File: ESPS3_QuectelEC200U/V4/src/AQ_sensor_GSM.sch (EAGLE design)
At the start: 160 parts, among them J1 F-1X03-SIP-100-32, J2 53261-0871, J3 PJ-002BH, J4 S8411-45R, Q2 MMBT2222, Q3 MMBT2222, Q4 MMBT2222, Q5 MMBT2222, Q6 MMBT2222, Q7 MMBT2222, Q8 FS8205, T1 S8050, T2 S8050, U1 CP2102N-A02-GQFN28, U2 DS1307Z, U5 TXS0108EPWR, X1 ESP32-S3-WROOM-1-N16R8, Y1 32.768kHz

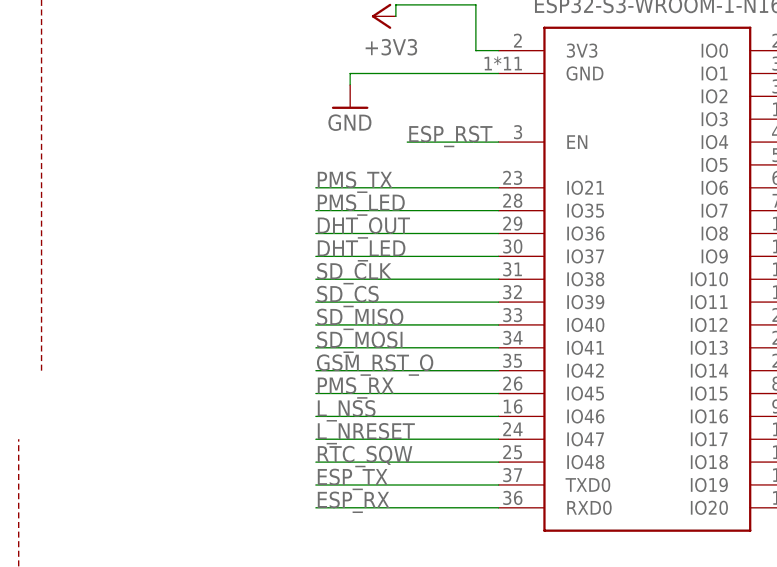
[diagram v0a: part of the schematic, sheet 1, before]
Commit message: V4 revised with images
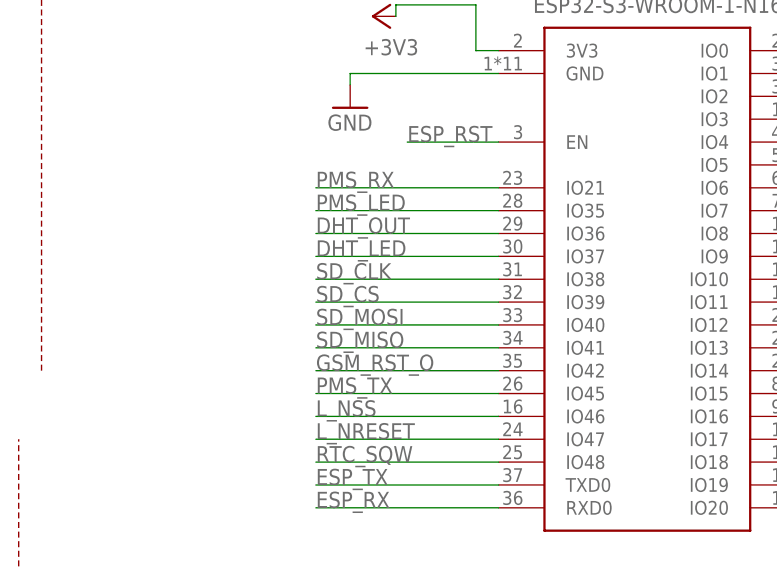
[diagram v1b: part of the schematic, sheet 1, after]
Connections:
- net PMS_RX: now also X1.IO21; no longer X1.IO45
- net PMS_TX: now also X1.IO45; no longer X1.IO21
- net SD_MISO: now also X1.IO41; no longer X1.IO40
- net SD_MOSI: now also X1.IO40; no longer X1.IO41
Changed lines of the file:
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@@
+</segment>
+<segment>
+<pinref part="X1" gate="G$1" pin="IO21"/>
+<wire x1="58.42" y1="147.32" x2="38.1" y2="147.32" width="0.1524" layer="91"/>
+<label x="38.1" y="147.32" size="1.778" layer="95"/>
+</segment>
+</net>
+<net name="PMS_TX" class="0">
+<segment>
+<pinref part="J2" gate="G$1" pin="4"/>
+<wire x1="322.58" y1="228.6" x2="309.88" y2="228.6" width="0.1524" layer="91"/>
+<label x="307.34" y="228.6" size="1.778" layer="95"/>
 </segment>
 <segment>
@@
 <wire x1="58.42" y1="124.46" x2="38.1" y2="124.46" width="0.1524" layer="91"/>
 <label x="38.1" y="124.46" size="1.778" layer="95"/>
-</segment>
-</net>
-<net name="PMS_TX" class="0">
-<segment>
-<pinref part="J2" gate="G$1" pin="4"/>
-<wire x1="322.58" y1="228.6" x2="309.88" y2="228.6" width="0.1524" layer="91"/>
-<label x="307.34" y="228.6" size="1.778" layer="95"/>
-</segment>
-<segment>
-<pinref part="X1" gate="G$1" pin="IO21"/>
-<wire x1="58.42" y1="147.32" x2="38.1" y2="147.32" width="0.1524" layer="91"/>
-<label x="38.1" y="147.32" size="1.778" layer="95"/>
 </segment>
 </net>
@@
 </segment>
 <segment>
+<pinref part="X1" gate="G$1" pin="IO40"/>
+<wire x1="58.42" y1="132.08" x2="38.1" y2="132.08" width="0.1524" layer="91"/>
+<label x="38.1" y="132.08" size="1.778" layer="95"/>
+</segment>
+</net>
+<net name="SD_CS" class="0">
+<segment>
+<pinref part="MICRO_SD1" gate="G$1" pin="CD/DAT3"/>
+<wire x1="58.42" y1="58.42" x2="45.72" y2="58.42" width="0.1524" layer="91"/>
+<label x="45.72" y="58.42" size="1.778" layer="95"/>
+</segment>
+<segment>
+<pinref part="X1" gate="G$1" pin="IO39"/>
+<wire x1="58.42" y1="134.62" x2="38.1" y2="134.62" width="0.1524" layer="91"/>
+<label x="38.1" y="134.62" size="1.778" layer="95"/>
+</segment>
+</net>
+<net name="SD_CLK" class="0">
+<segment>
+<pinref part="MICRO_SD1" gate="G$1" pin="CLK"/>
+<wire x1="58.42" y1="73.66" x2="45.72" y2="73.66" width="0.1524" layer="91"/>
+<label x="45.72" y="73.66" size="1.778" layer="95"/>
+</segment>
+<segment>
+<pinref part="X1" gate="G$1" pin="IO38"/>
+<wire x1="58.42" y1="137.16" x2="38.1" y2="137.16" width="0.1524" layer="91"/>
+<label x="38.1" y="137.16" size="1.778" layer="95"/>
+</segment>
+</net>
+<net name="SD_MISO" class="0">
+<segment>
+<pinref part="MICRO_SD1" gate="G$1" pin="CMD"/>
+<wire x1="58.42" y1="71.12" x2="35.56" y2="71.12" width="0.1524" layer="91"/>
+<label x="35.56" y="71.12" size="1.778" layer="95"/>
+</segment>
+<segment>
 <pinref part="X1" gate="G$1" pin="IO41"/>
 <wire x1="58.42" y1="129.54" x2="38.1" y2="129.54" width="0.1524" layer="91"/>
@@
 </segment>
 </net>
-<net name="SD_CS" class="0">
-<segment>
-<pinref part="MICRO_SD1" gate="G$1" pin="CD/DAT3"/>
-<wire x1="58.42" y1="58.42" x2="45.72" y2="58.42" width="0.1524" layer="91"/>
-<label x="45.72" y="58.42" size="1.778" layer="95"/>
-</segment>
-<segment>
-<pinref part="X1" gate="G$1" pin="IO39"/>
-<wire x1="58.42" y1="134.62" x2="38.1" y2="134.62" width="0.1524" layer="91"/>
-<label x="38.1" y="134.62" size="1.778" layer="95"/>
-</segment>
-</net>
-<net name="SD_CLK" class="0">
-<segment>
-<pinref part="MICRO_SD1" gate="G$1" pin="CLK"/>
-<wire x1="58.42" y1="73.66" x2="45.72" y2="73.66" width="0.1524" layer="91"/>
-<label x="45.72" y="73.66" size="1.778" layer="95"/>
-</segment>
-<segment>
-<pinref part="X1" gate="G$1" pin="IO38"/>
-<wire x1="58.42" y1="137.16" x2="38.1" y2="137.16" width="0.1524" layer="91"/>
-<label x="38.1" y="137.16" size="1.778" layer="95"/>
-</segment>
-</net>
-<net name="SD_MISO" class="0">
-<segment>
-<pinref part="MICRO_SD1" gate="G$1" pin="CMD"/>
-<wire x1="58.42" y1="71.12" x2="35.56" y2="71.12" width="0.1524" layer="91"/>
-<label x="35.56" y="71.12" size="1.778" layer="95"/>
-</segment>
-<segment>
-<pinref part="X1" gate="G$1" pin="IO40"/>
-<wire x1="58.42" y1="132.08" x2="38.1" y2="132.08" width="0.1524" layer="91"/>
-<label x="38.1" y="132.08" size="1.778" layer="95"/>
-</segment>
-</net>
